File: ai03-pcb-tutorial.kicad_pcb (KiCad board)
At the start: 2 copper layers, 77.4 x 39.5 mm, 24 parts, among them SW1 SW_PUSH, U1 ATmega32U4-AU, Y1 16MHz

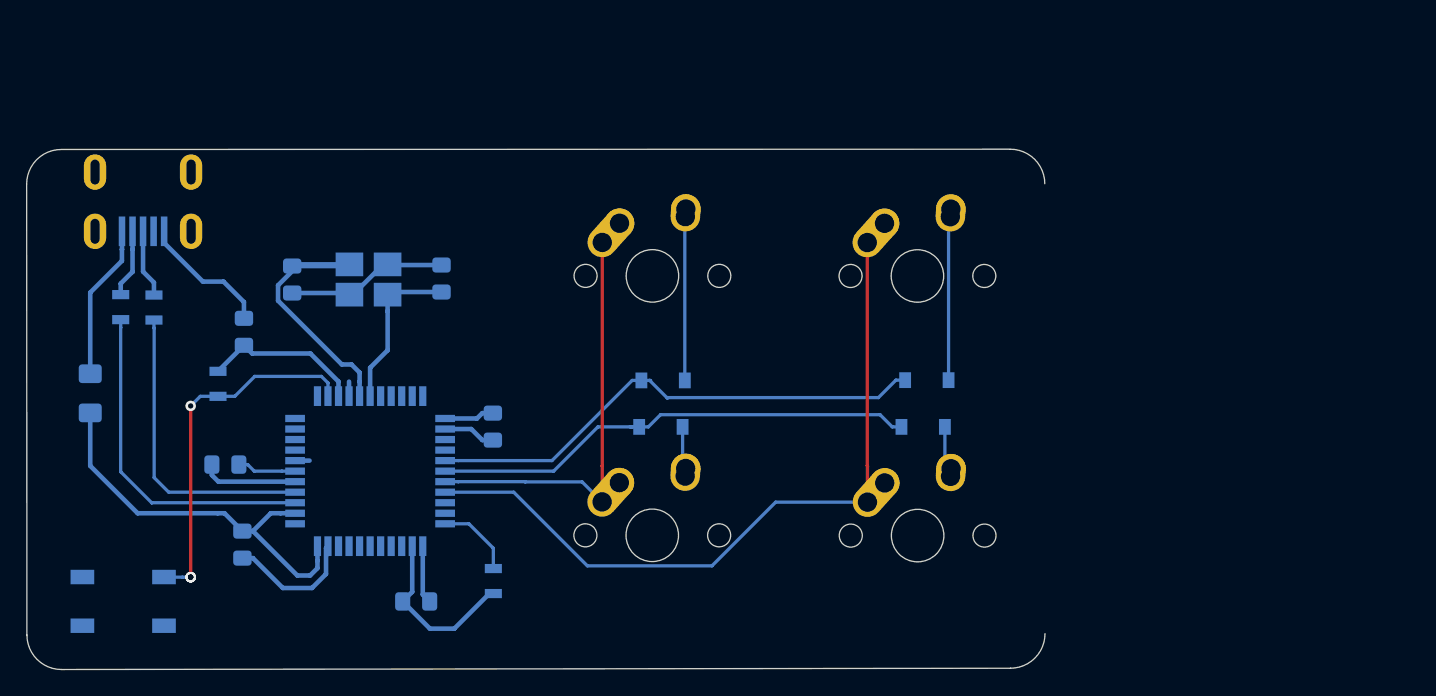
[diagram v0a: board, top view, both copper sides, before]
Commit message: reset edge line
reset edge line
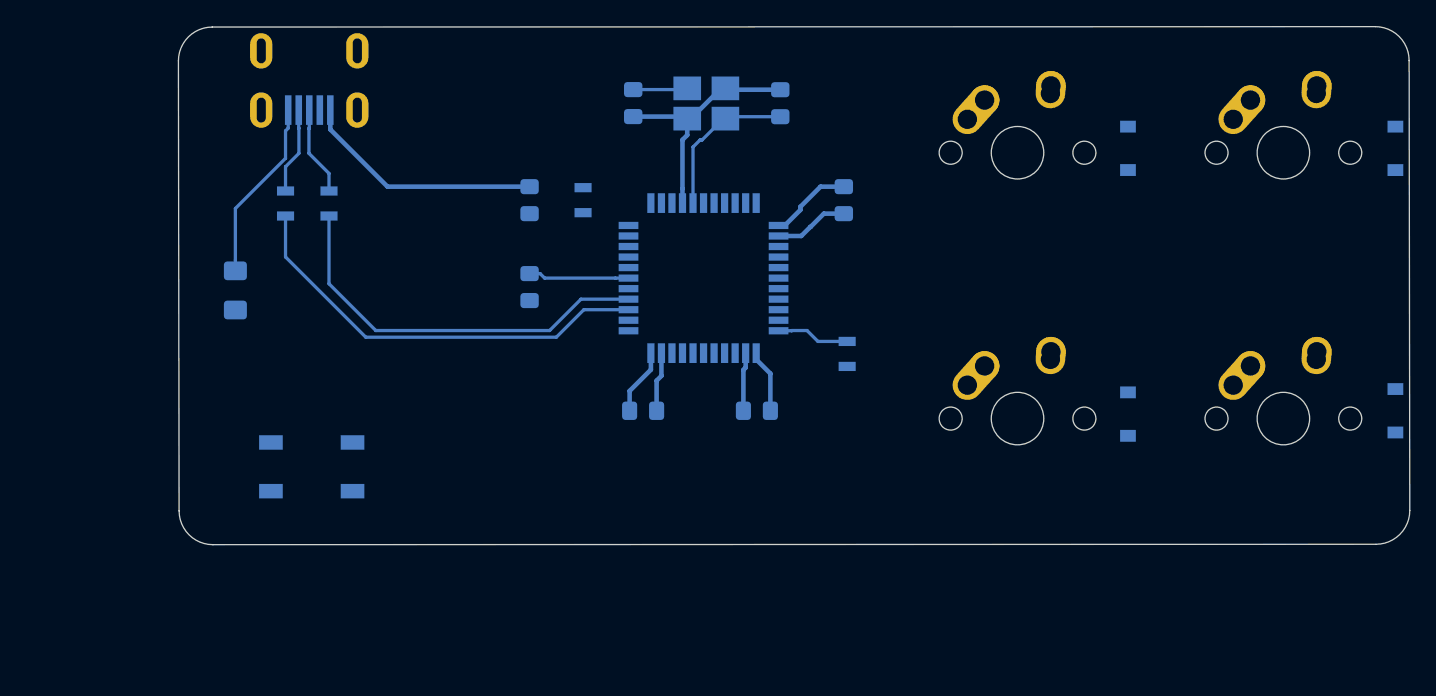
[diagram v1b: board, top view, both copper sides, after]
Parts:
- moved D3 59.7 mm to (116.3, 62.6), turned to 90 degrees
- moved MX3 56.1 mm to (107.8, 62.9)
- moved C5 52.7 mm to (74.4, 66.5), turned to 90 degrees
- moved C2 39.4 mm to (69.6, 59.2), turned to 270 degrees
- moved D4 35.9 mm to (116.3, 82.5), turned to 90 degrees
- moved D1 35.4 mm to (96.0, 82.8), turned to 90 degrees
- moved R4 31.9 mm to (74.7, 78.2)
- moved R1 31.0 mm to (54.6, 66.5), turned to 270 degrees
- moved MX1 29.8 mm to (87.6, 83.1)
- moved U1 29.3 mm to (63.8, 72.5)
- moved MX4 29.2 mm to (107.8, 83.1)
- moved Y1 28.9 mm to (64.0, 59.2), turned to 0 degrees
- moved C3 26.8 mm to (50.5, 73.2), turned to 270 degrees
- moved C4 23.9 mm to (50.5, 66.5)
- moved D2 23.3 mm to (96.0, 62.6), turned to 90 degrees
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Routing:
- net COL1: track 56.2 -> 0.00 mm
- net ROW0: track 38.7 -> 0.00 mm
- net ROW1: track 37.0 -> 0.00 mm
- net +5V: track 52.1 -> 15.5 mm
- net COL0: track 32.3 -> 0.00 mm
- net Net-(R1-Pad1): track 27.6 -> 0.00 mm, vias 4 -> 0
- net Net-(D2-Pad2): track 13.1 -> 0.00 mm
- net Net-(D1-Pad2): track 12.5 -> 0.00 mm
- net Net-(C2-Pad2): track 21.9 -> 11.8 mm
- net Net-(C1-Pad2): track 12.4 -> 4.14 mm
- net Net-(R2-Pad1): track 23.1 -> 30.4 mm
- net Net-(R3-Pad1): track 25.8 -> 32.6 mm
- net GND: track 58.5 -> 52.5 mm
- net Net-(D3-Pad2): track 3.82 -> 0.00 mm
- net Net-(D4-Pad2): track 3.37 -> 0.00 mm
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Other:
- board size 77.4 x 39.5 mm -> 93.6 x 39.4 mm
